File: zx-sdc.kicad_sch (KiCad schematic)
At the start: 65 parts, among them J1 SD_Card, J2 Micro_SD_Card_Det2, J3 Conn_01x02_Pin, Q1 2N7000, Q2 BC557, U1 74LS688, U10 74LS125, U11 74LS595, U12 74LS30, U13 74LS138, U2 74LS139, U3 AMS1117-3.3, U4 74LS166, U5 74LS595, U6 74LS04, U7 74LS163, U8 74LS74, U9 74LS74, Y1 8MHz

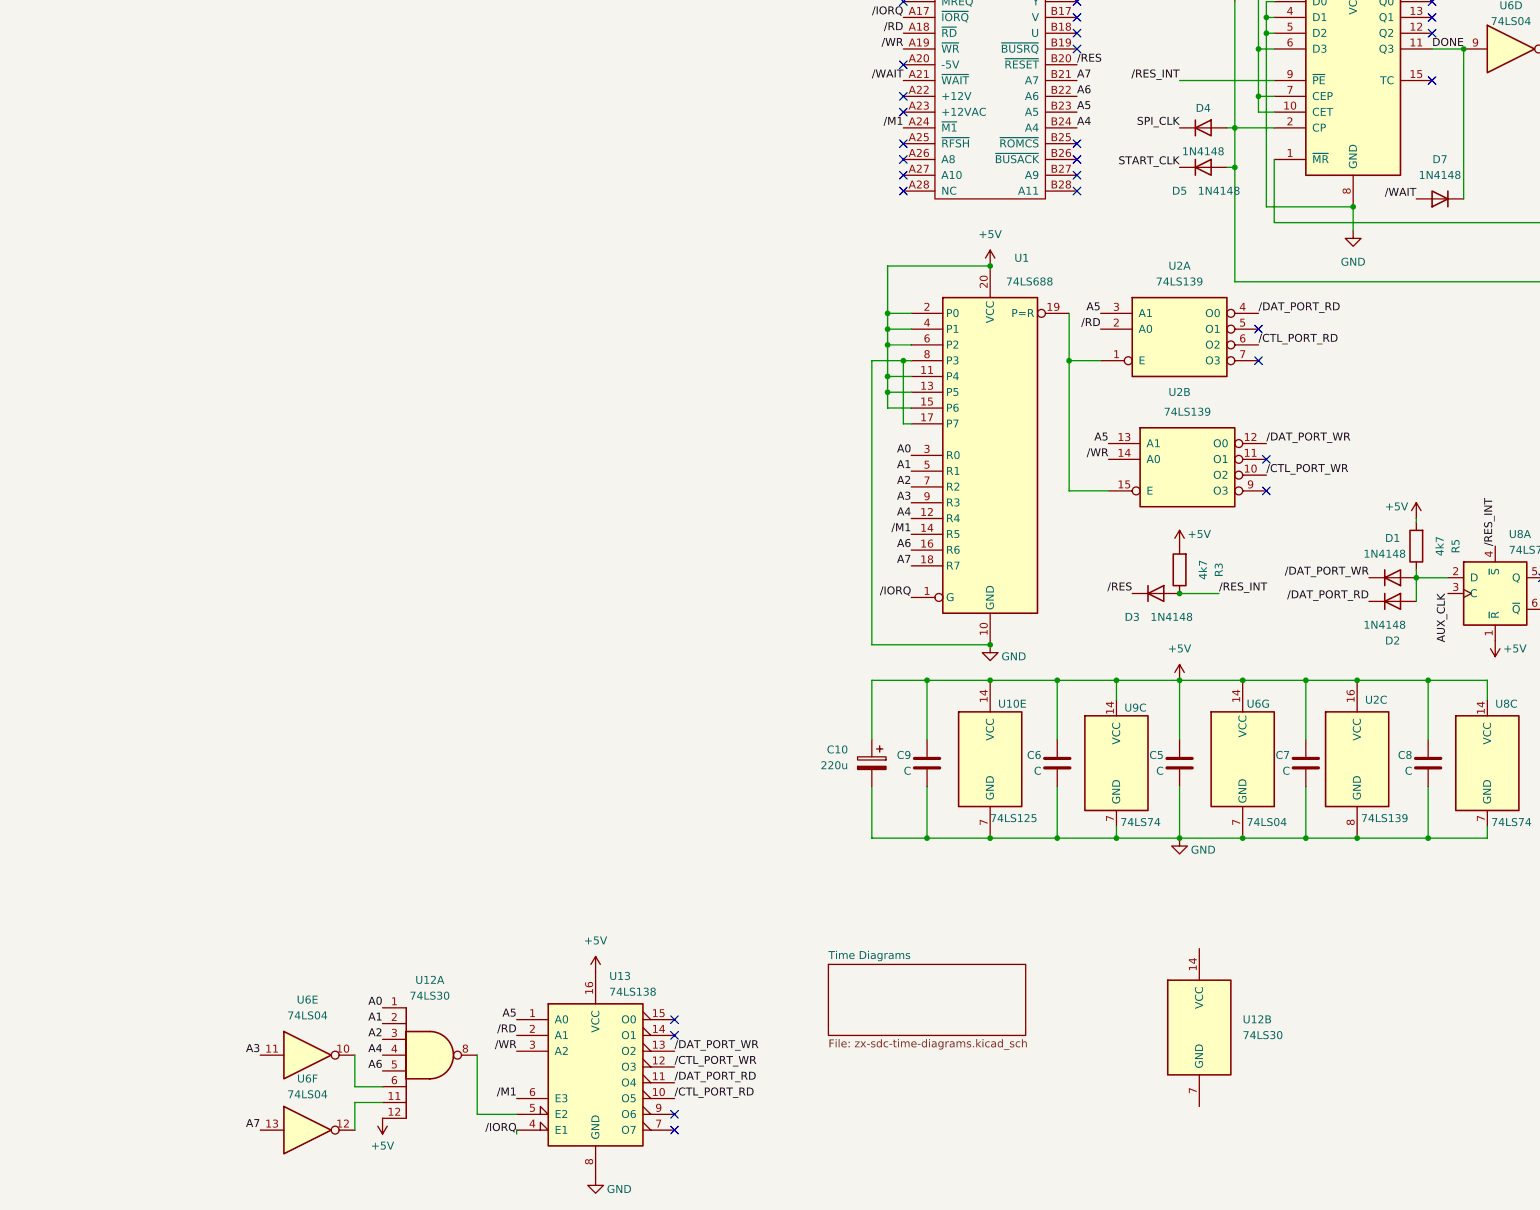
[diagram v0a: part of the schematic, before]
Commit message: preparation for board design
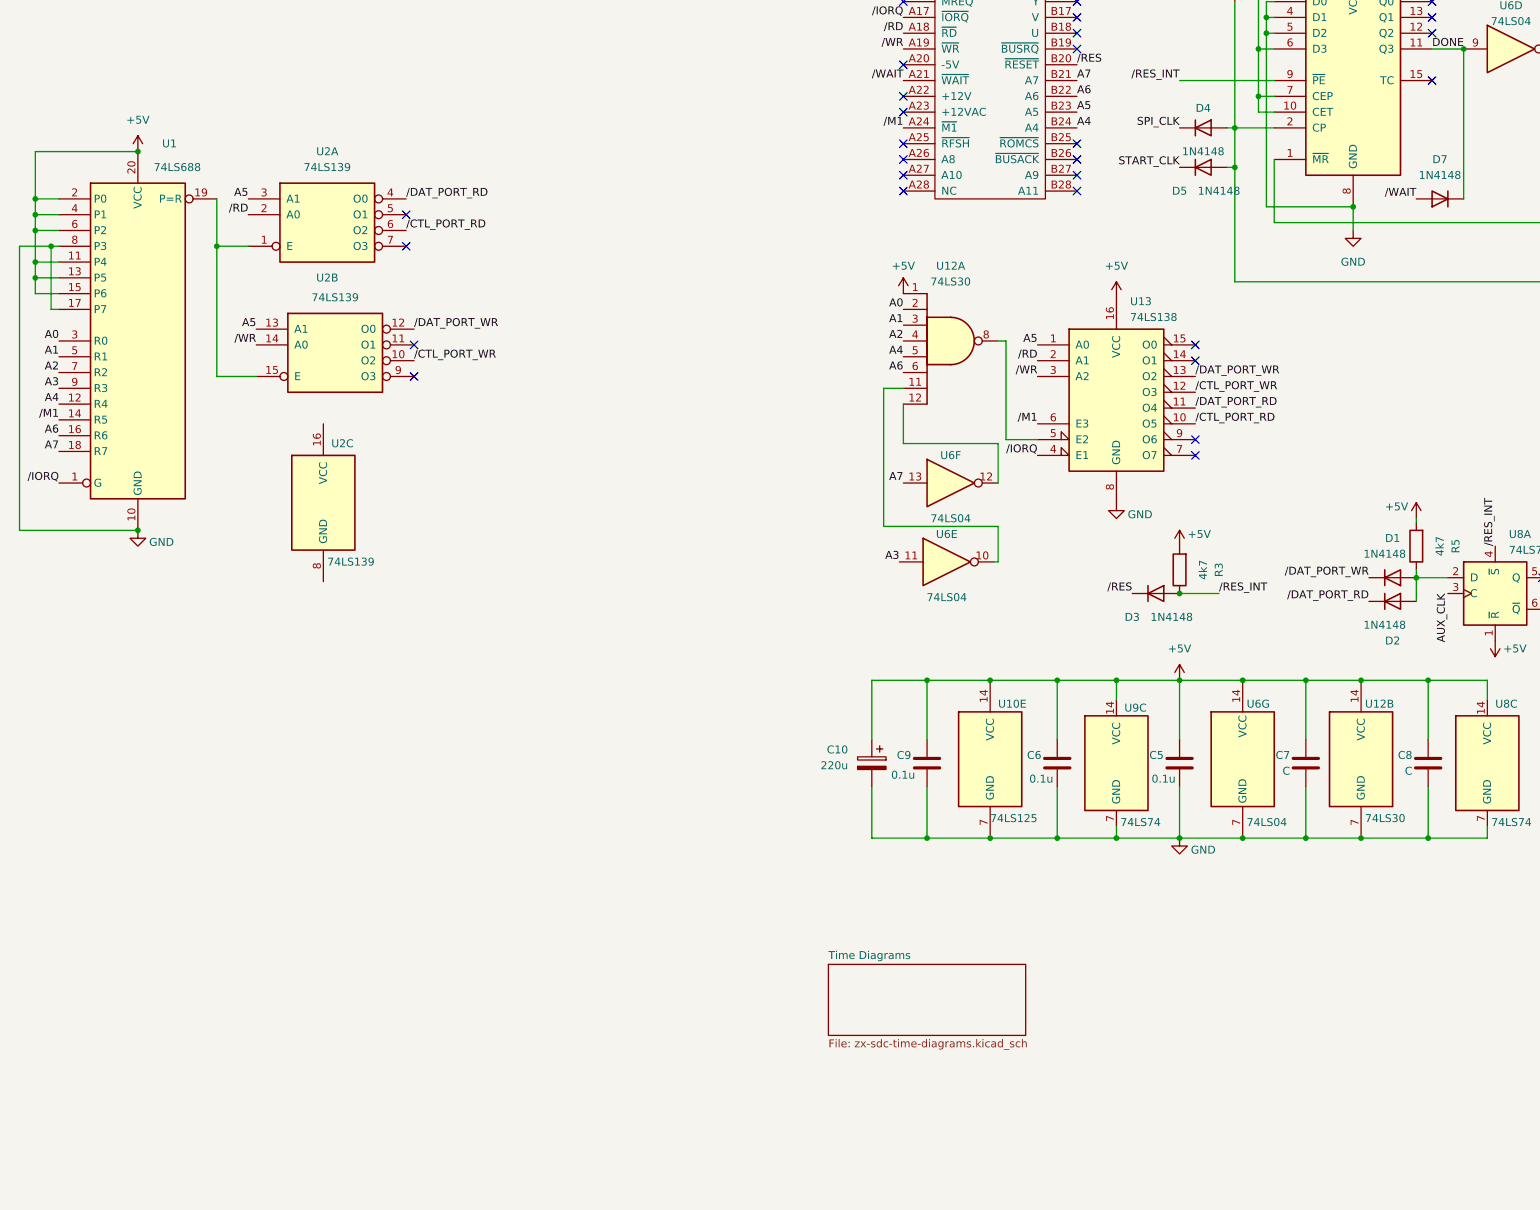
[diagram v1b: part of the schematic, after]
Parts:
- C5, C6, C9: value C -> 0.1u
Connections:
- net +5V: now also U12.1, U12.14 (VCC); no longer U12.12, U2.16 (VCC)
- net A0: now also U12.2; no longer U12.1
- net A1: now also U12.3; no longer U12.2
- net A2: now also U12.4; no longer U12.3
- net A4: now also U12.5; no longer U12.4
- net A6: now also U12.6; no longer U12.5
- net GND: now also U12.7 (GND); no longer U2.8 (GND)
- net at U12.11: now also U6.10; no longer U6.12
- new net: U12.12, U6.12
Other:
- moved on the sheet: U1, U12A, U12B, U13, U2A, U2B, U6E, U6F
